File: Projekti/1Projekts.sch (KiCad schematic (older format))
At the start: 11 parts

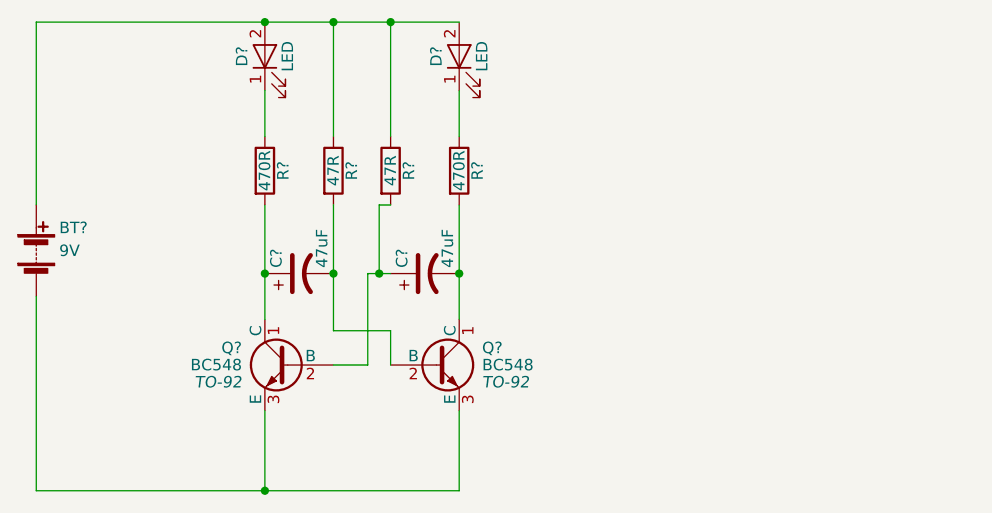
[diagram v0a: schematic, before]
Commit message: pievienojaam lib jaunu kompunenti
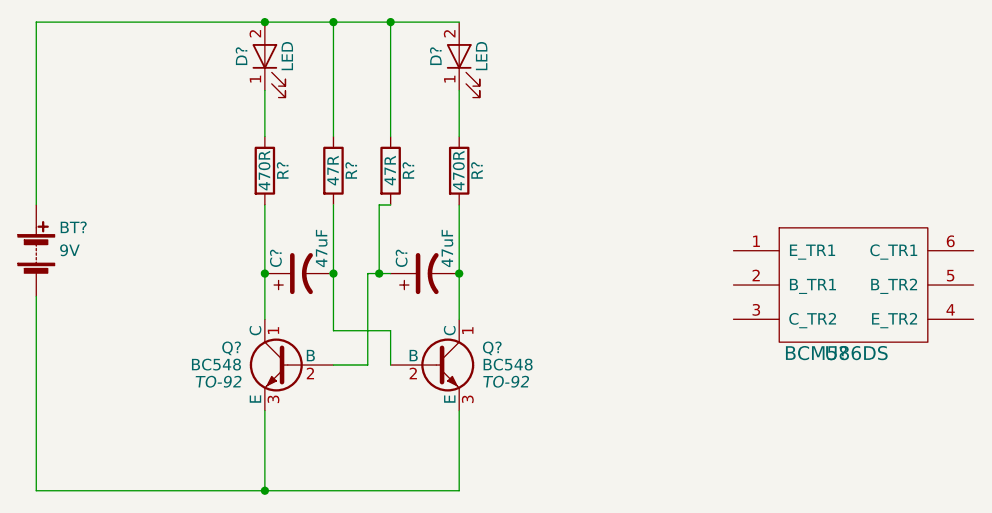
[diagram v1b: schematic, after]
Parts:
- added U?: BCM586DS, symbol BCM586DS
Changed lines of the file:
@@
 EESchema Schematic File Version 2
+LIBS:BCM
 LIBS:power
 LIBS:device
@@
 LIBS:contrib
 LIBS:valves
+LIBS:1Projekts-cache
 EELAYER 25 0
 EELAYER END
@@
 	5850 3500 5900 3500
 Connection ~ 5850 3800
+$Comp
+L BCM586DS U?
+U 1 1 58C14A42
+P 7800 4000
+F 0 "U?" H 7850 3850 60  0000 C CNN
+F 1 "BCM586DS" H 7850 3850 60  0000 C CNN
+F 2 "" H 7850 3850 60  0001 C CNN
+F 3 "" H 7850 3850 60  0001 C CNN
+	1    7800 4000
+	1    0    0    -1
+$EndComp
 $EndSCHEMATC
